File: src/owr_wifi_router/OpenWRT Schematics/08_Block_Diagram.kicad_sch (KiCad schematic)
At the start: 1 part

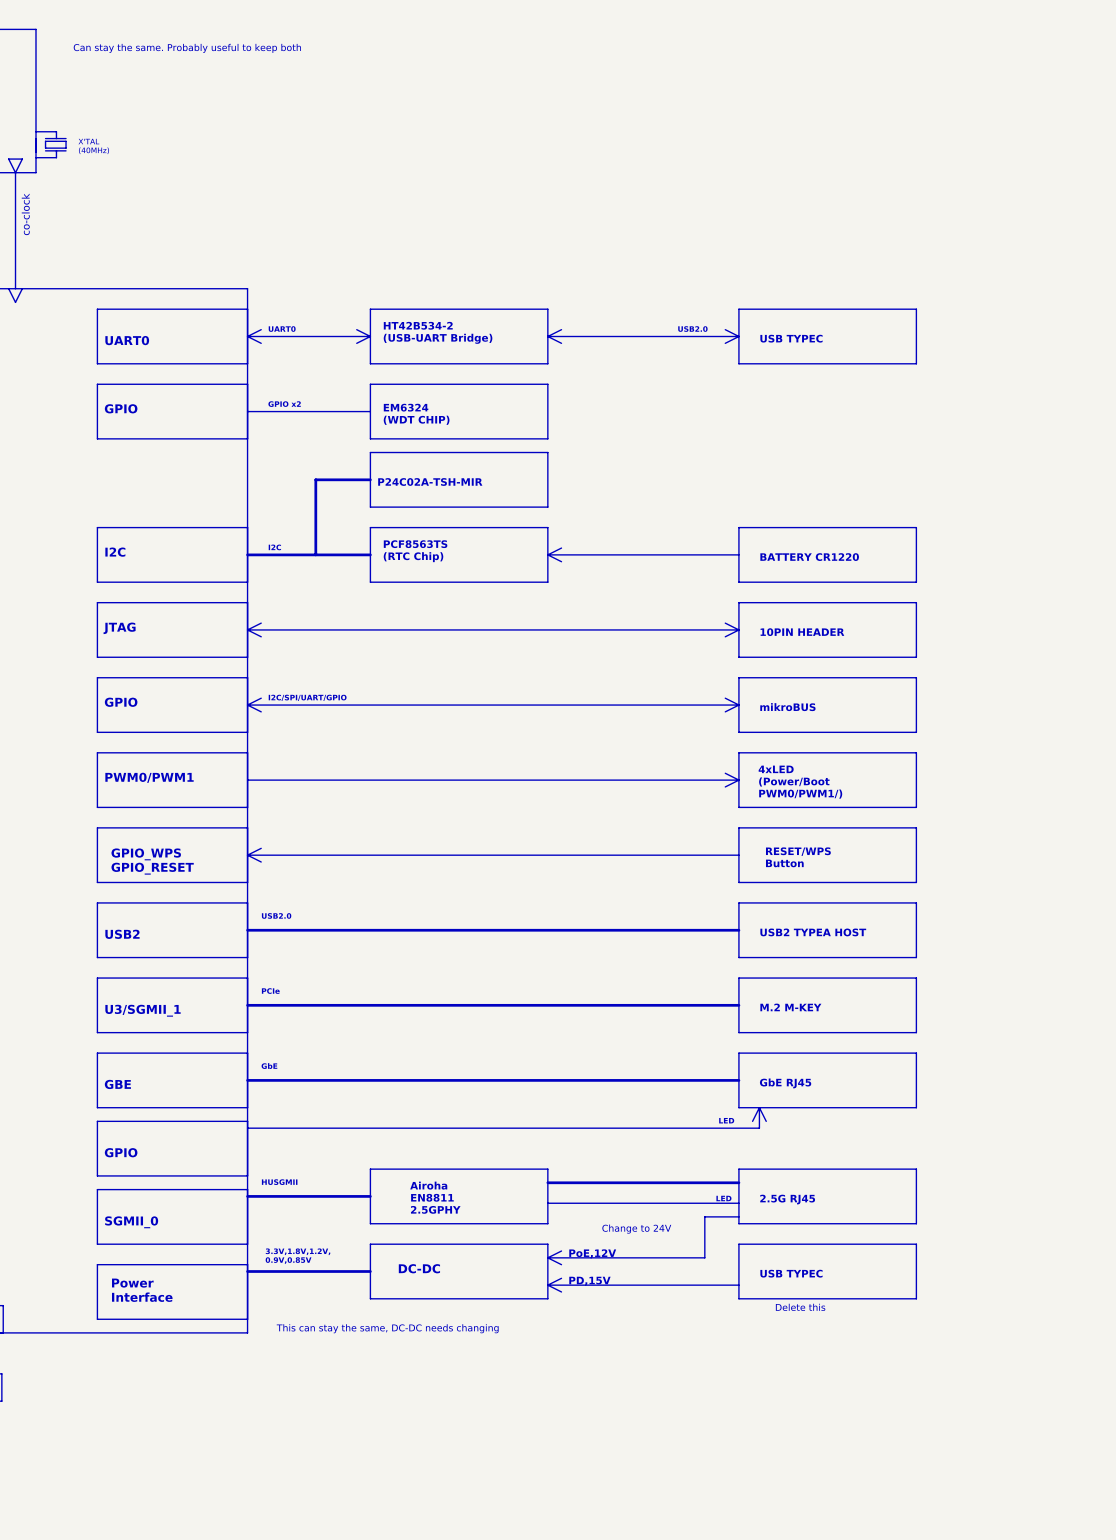
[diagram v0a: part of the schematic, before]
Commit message: Began work on DC-DC
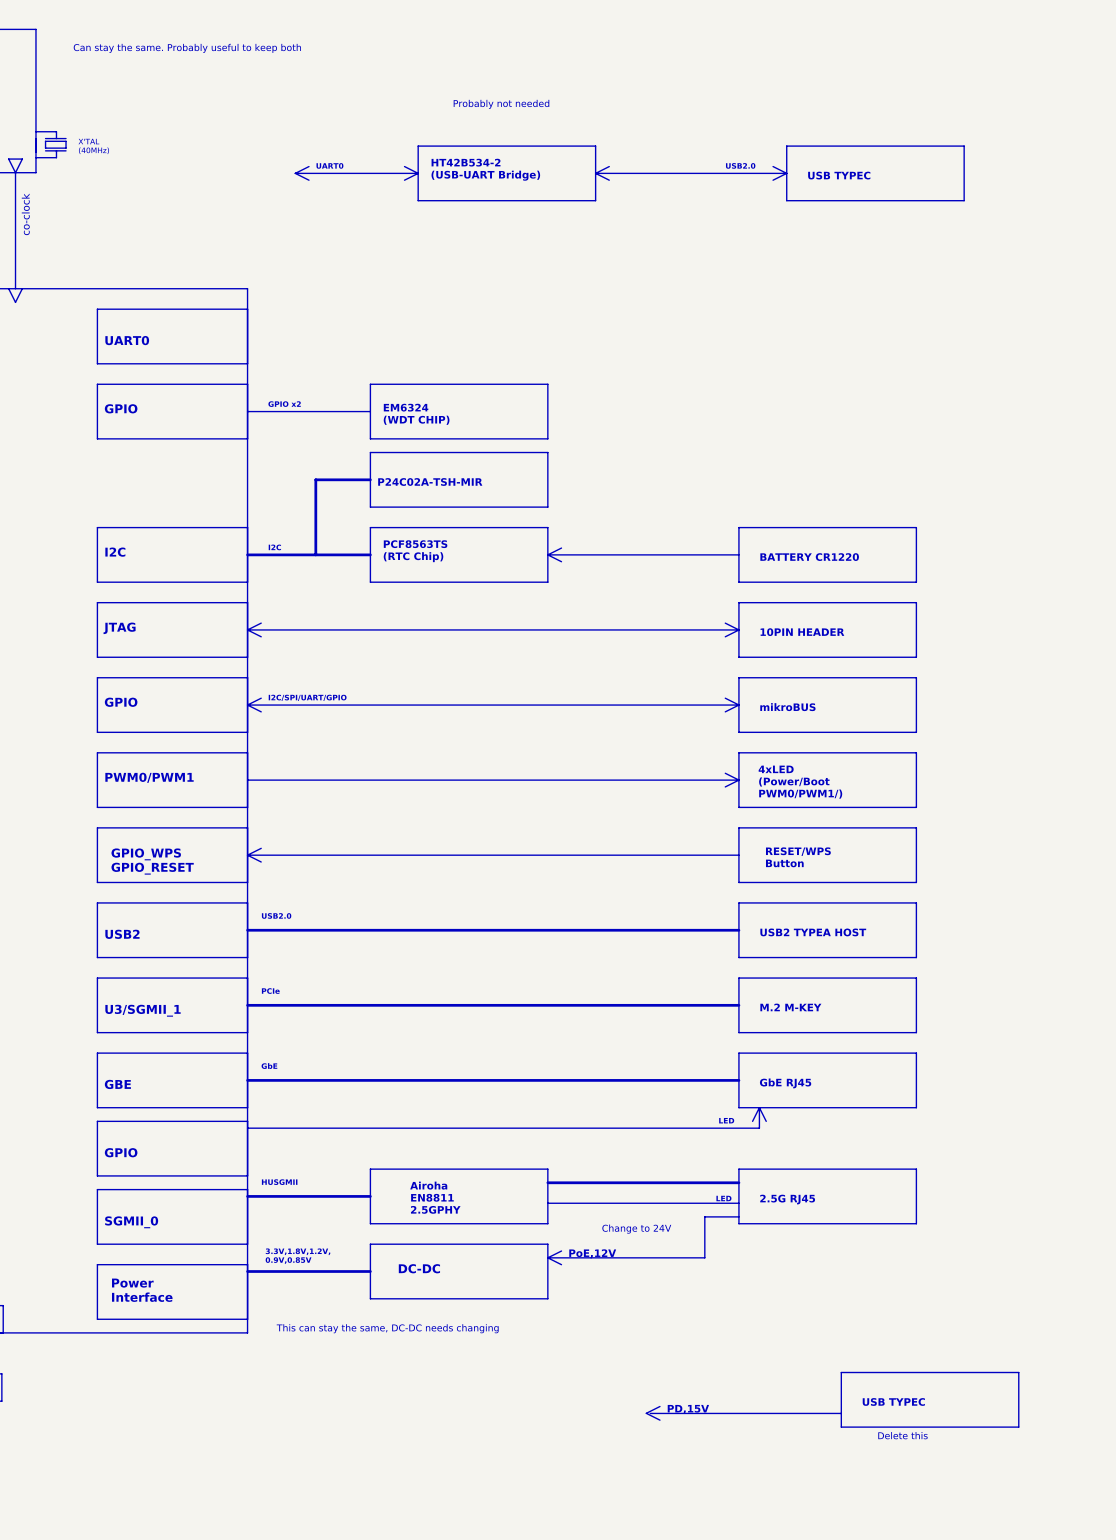
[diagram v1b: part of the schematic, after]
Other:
- note added: "Probably not needed"
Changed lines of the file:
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@@
 	)
 	(rectangle
-		(start 462.28 135.509)
-		(end 429.26 145.669)
+		(start 471.17 105.156)
+		(end 438.15 115.316)
 		(stroke
 			(width 0.254)
@@
 	)
 	(rectangle
-		(start 393.7 135.509)
-		(end 360.68 145.669)
+		(start 402.59 105.156)
+		(end 369.57 115.316)
 		(stroke
 			(width 0.254)
@@
 	)
 	(rectangle
-		(start 337.82 299.339)
-		(end 309.88 309.499)
+		(start 309.88 299.339)
+		(end 337.82 309.499)
 		(stroke
 			(width 0.254)
@@
 	)
 	(rectangle
-		(start 429.26 309.499)
-		(end 462.28 319.659)
+		(start 448.31 333.375)
+		(end 481.33 343.535)
 		(stroke
 			(width 0.254)
@@
 	)
 	(rectangle
-		(start 337.82 204.089)
-		(end 309.88 214.249)
+		(start 309.88 204.089)
+		(end 337.82 214.249)
 		(stroke
 			(width 0.254)
@@
 	)
 	(rectangle
-		(start 337.82 273.939)
-		(end 309.88 284.099)
+		(start 309.88 273.939)
+		(end 337.82 284.099)
 		(stroke
 			(width 0.254)
@@
 	(text "PD,15V"
 		(exclude_from_sim no)
-		(at 397.51 317.373 0)
+		(at 415.8332 341.2265 0)
 		(effects
 			(font
@@
 	(text "USB2.0"
 		(exclude_from_sim no)
-		(at 417.83 140.081 0)
+		(at 426.72 109.728 0)
 		(effects
 			(font
@@
 	(text "Delete this\n"
 		(exclude_from_sim no)
-		(at 440.69 321.564 0)
+		(at 459.74 345.44 0)
 		(effects
 			(font
@@
 	(text "USB TYPEC"
 		(exclude_from_sim no)
-		(at 433.07 142.113 0)
+		(at 441.96 111.76 0)
 		(effects
 			(font
@@
 		)
 	)
+	(text "Probably not needed\n"
+		(exclude_from_sim no)
+		(at 385.064 97.536 0)
+		(effects
+			(font
+				(size 1.27 1.27)
+			)
+		)
+	)
 	(text "JTAG"
 		(exclude_from_sim no)
@@
 	(text "USB TYPEC"
 		(exclude_from_sim no)
-		(at 433.07 316.103 0)
+		(at 452.12 339.979 0)
 		(effects
 			(font
@@
 	(text "UART0"
 		(exclude_from_sim no)
-		(at 341.63 140.081 0)
+		(at 350.52 109.728 0)
 		(effects
 			(font
@@
 	(text_box "Airoha\nEN8811\n2.5GPHY"
 		(exclude_from_sim no)
-		(at 380.238 305.181 0)
-		(size -13.208 -8.382)
+		(at 367.03 296.799 0)
+		(size 13.208 8.382)
 		(margins 1.0477 1.0477 1.0477 1.0477)
 		(stroke
@@
 	(text_box "PCF8563TS\n(RTC Chip)"
 		(exclude_from_sim no)
-		(at 380.492 183.007 0)
-		(size -18.542 -5.588)
+		(at 361.95 177.419 0)
+		(size 18.542 5.588)
 		(margins 1.0477 1.0477 1.0477 1.0477)
 		(stroke
@@
 	(text_box "PHY0\nWRI"
 		(exclude_from_sim no)
-		(at 181.864 140.081 0)
-		(size -9.144 -7.112)
+		(at 172.72 132.969 0)
+		(size 9.144 7.112)
 		(margins 1.2382 1.2382 1.2382 1.2382)
 		(stroke
@@
 	(text_box "HT42B534-2\n(USB-UART Bridge)"
 		(exclude_from_sim no)
-		(at 392.938 142.367 0)
-		(size -30.988 -5.588)
+		(at 370.84 106.426 0)
+		(size 30.988 5.588)
 		(margins 1.0477 1.0477 1.0477 1.0477)
 		(stroke
@@
 	(polyline
 		(pts
-			(xy 396.24 315.849) (xy 393.7 317.119)
+			(xy 414.5632 339.7025) (xy 412.0232 340.9725)
 		)
 		(stroke
@@
 	(polyline
 		(pts
-			(xy 396.24 141.859) (xy 393.7 140.589)
+			(xy 405.13 111.506) (xy 402.59 110.236)
 		)
 		(stroke
@@
 	(polyline
 		(pts
-			(xy 340.36 139.319) (xy 337.82 140.589)
+			(xy 349.25 108.966) (xy 346.71 110.236)
 		)
 		(stroke
@@
 	(polyline
 		(pts
-			(xy 337.82 140.589) (xy 360.68 140.589)
+			(xy 346.71 110.236) (xy 369.57 110.236)
 		)
 		(stroke
@@
 	(polyline
 		(pts
-			(xy 358.14 141.859) (xy 360.68 140.589)
+			(xy 367.03 111.506) (xy 369.57 110.236)
 		)
 		(stroke
@@
 	(polyline
 		(pts
-			(xy 340.36 141.859) (xy 337.82 140.589)
+			(xy 349.25 111.506) (xy 346.71 110.236)
 		)
 		(stroke
@@
 	(polyline
 		(pts
-			(xy 426.72 139.319) (xy 429.26 140.589)
+			(xy 435.61 108.966) (xy 438.15 110.236)
 		)
 		(stroke
@@
 	(polyline
 		(pts
-			(xy 426.72 141.859) (xy 429.26 140.589)
+			(xy 435.61 111.506) (xy 438.15 110.236)
 		)
 		(stroke
@@
 	(polyline
 		(pts
-			(xy 393.7 140.589) (xy 429.26 140.589)
+			(xy 402.59 110.236) (xy 438.15 110.236)
 		)
 		(stroke
@@
 	(polyline
 		(pts
-			(xy 393.7 317.119) (xy 429.26 317.119)
+			(xy 412.75 340.995) (xy 448.31 340.995)
 		)
 		(stroke
@@
 	(polyline
 		(pts
-			(xy 358.14 139.319) (xy 360.68 140.589)
+			(xy 367.03 108.966) (xy 369.57 110.236)
 		)
 		(stroke
@@
 	(polyline
 		(pts
-			(xy 396.24 139.319) (xy 393.7 140.589)
+			(xy 405.13 108.966) (xy 402.59 110.236)
 		)
 		(stroke
@@
 	(polyline
 		(pts
-			(xy 396.24 318.389) (xy 393.7 317.119)
-		)
-		(stroke
+			(xy 414.5632 342.2425) (xy 412.0232 340.9725)
+		)
+		(stroke
